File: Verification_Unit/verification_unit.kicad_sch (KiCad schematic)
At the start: 35 parts, among them J1 Conn_02x04_Counter_Clockwise, M1 Motor_DC, Q2 2N3055, U1 STM32C011F4Px, U2 L293D, U3 CC1101RGPR, U4 LM3940IT-3.3, U6 LM741, Y1 NX3225GA-26.000MHZ-EXS00A-CG0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

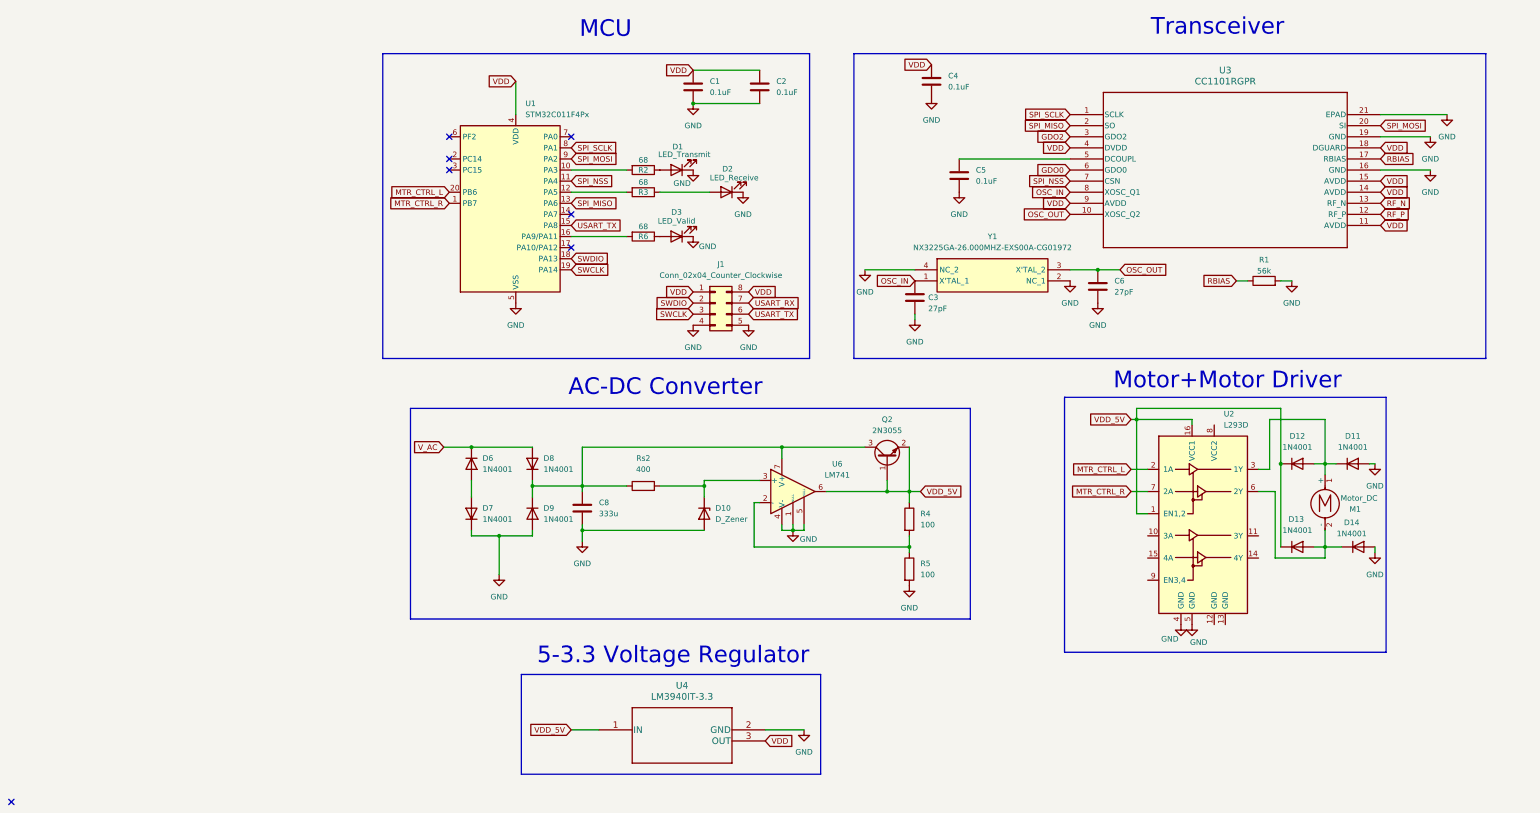
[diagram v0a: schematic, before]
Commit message: bruh
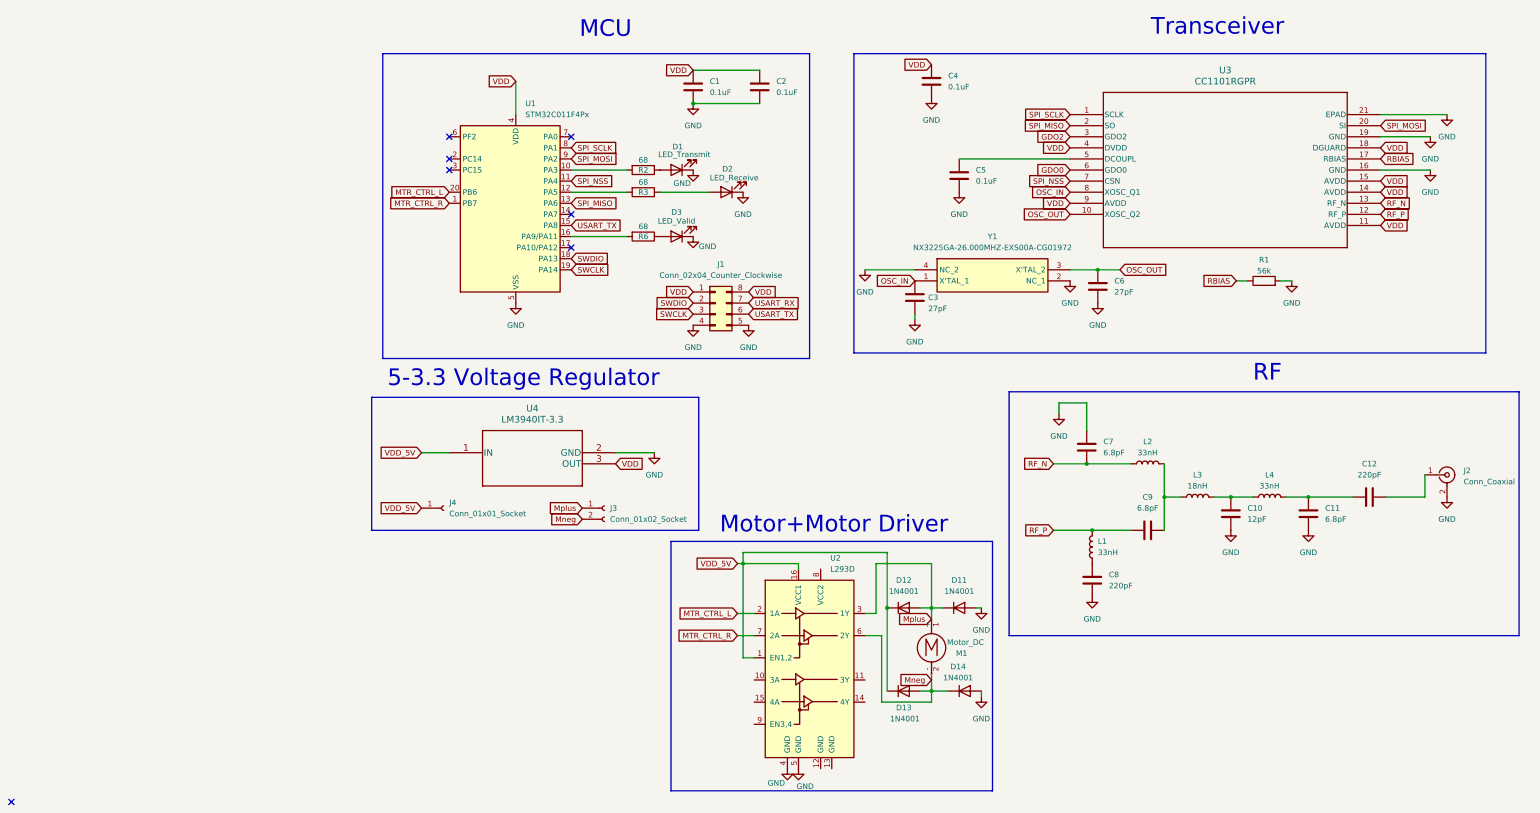
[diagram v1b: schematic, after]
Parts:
- removed D10: D_Zener, symbol Device:D_Zener
- removed D6, D7, D8, D9: 1N4001, Diode_THT:D_DO-41_SOD81_P10.16mm_Horizontal, symbol Diode:1N4001
- removed Q2: 2N3055, Package_TO_SOT_THT:TO-3, symbol Transistor_BJT:2N3055
- removed R4, R5: 100, symbol Device:R
- removed Rs2: 400, symbol Device:R
- removed U6: LM741, symbol Amplifier_Operational:LM741
- added C10: 12pF, Capacitor_SMD:C_0805_2012Metric, symbol Device:C
- added C11, C7, C9: 6.8pF, Capacitor_SMD:C_0805_2012Metric, symbol Device:C
- added C12: 220pF, Capacitor_SMD:C_0805_2012Metric, symbol Device:C
- added J2: Conn_Coaxial, Connector_Coaxial:SMA_Amphenol_901-143_Horizontal, symbol Connector:Conn_Coaxial
- added J3: Conn_01x02_Socket, Connector_PinSocket_2.54mm:PinSocket_1x02_P2.54mm_Vertical, symbol Connector:Conn_01x02_Socket
- added J4: Conn_01x01_Socket, Connector_PinSocket_2.54mm:PinSocket_1x01_P2.54mm_Vertical, symbol Connector:Conn_01x01_Socket
- added L1, L2, L4: 33nH, Inductor_SMD:L_0805_2012Metric, symbol Device:L
- added L3: 18nH, Inductor_SMD:L_0805_2012Metric, symbol Device:L
- C1, C2, C4, C5: footprint Capacitor_SMD:C_0603_1608Metric -> Capacitor_SMD:C_0805_2012Metric
- C3, C6: footprint Capacitor_SMD:C_0402_1005Metric -> Capacitor_SMD:C_0805_2012Metric
- C8: value 333u -> 220pF; footprint (none) -> Capacitor_SMD:C_0805_2012Metric
- D1, D2, D3: footprint (none) -> LED_SMD:LED_0805_2012Metric
- D11, D12, D13, D14: footprint Diode_THT:D_DO-41_SOD81_P10.16mm_Horizontal -> Diode_SMD:D_0805_2012Metric
- R1: footprint Resistor_SMD:R_0402_1005Metric -> Capacitor_SMD:C_0805_2012Metric
- R2, R3, R6: footprint (none) -> Resistor_SMD:R_0805_2012Metric
- U3: footprint CC1101:RGP20_2P4X2P4 -> newparts:RGP20_2P4X2P4
- U4: footprint T03B -> newparts:LM3940IT-3.3
- Y1: footprint SamacSys_Parts:NX3225GA16000MSTDCRG1 -> newparts:NX3225GA16000MSTDCRG1
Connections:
- net GND: now also C8.1, C10.1, C11.1, C7.2, J2.2 (Ext); no longer C8.2
- net RF_N: now also C7.1, L2.1
- net RF_P: now also C9.2, L1.2
- net VDD_5V: now also J4.1 (Pin_1)
- net Mneg: now reaches D13.2 (A), D14.1 (K), M1.2 (-), U2.6 (2Y)
- net Mneg: now also J3.2 (Pin_2)
- net Mplus: now reaches D11.1 (K), D12.2 (A), M1.1 (+), U2.3 (1Y)
- net Mplus: now also J3.1 (Pin_1)
- new net: C9.1, L2.2, L3.1
- new net: C10.2, L3.2, L4.1
- new net: C8.2, L1.1
- new net: C11.2, C12.1, L4.2
- new net: C12.2, J2.1 (In)
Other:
- note added: "RF"
- note removed: "AC-DC Converter"
- moved on the sheet: D11, D12, D13, D14, M1, U2, U4
